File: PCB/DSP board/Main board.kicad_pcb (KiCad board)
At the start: 4 copper layers, 60 x 100 mm, 208 parts, among them J201 01x06 male SMD, J701 Conn_01x40_Female, J702 Conn_01x06_Female, J801 1140084168, J901 USB_B, U201 STM32H743II, U401 AS4C32M8SA, U501 CS42448, U601 MIC23050, U602 TPS2113A, U603 TPS61170, U604 ADP150, U901 USB3300-EZK, X101 Mini_PCI-e, Y201 ABS05-32.768, Y202 CX2016DB16000, Y901 XRCGB24M000F1H02R0

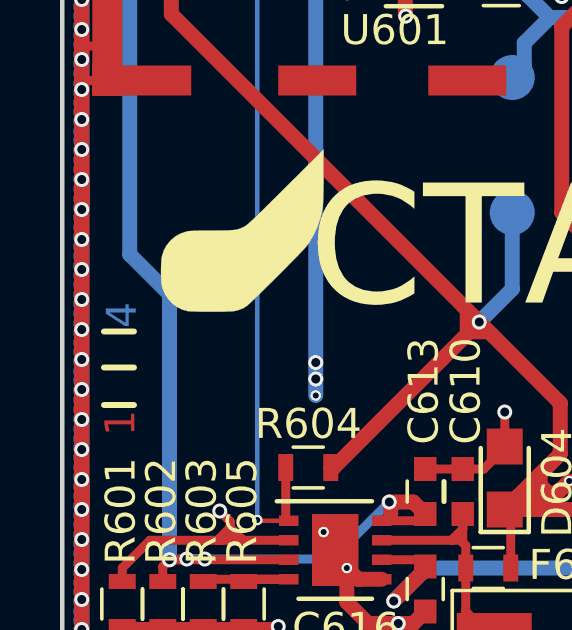
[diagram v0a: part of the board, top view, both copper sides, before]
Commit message: Minor updates keepout
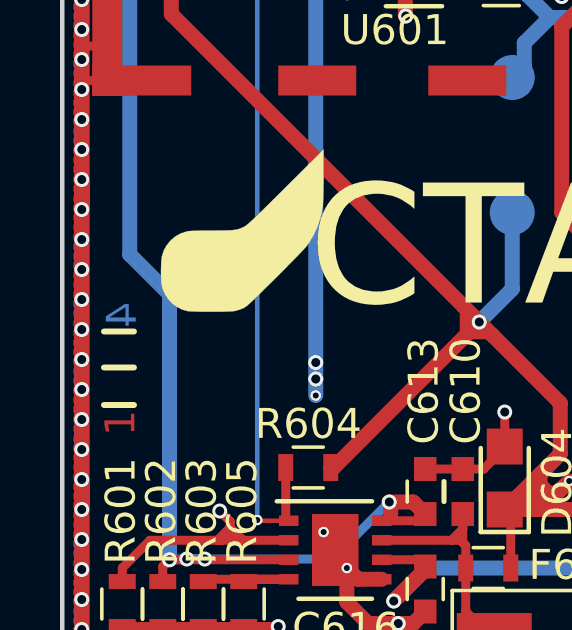
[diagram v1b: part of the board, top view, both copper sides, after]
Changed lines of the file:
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@@
   (layers
     (0 F.Cu mixed)
-    (1 In1.Cu mixed hide)
+    (1 In1.Cu mixed)
     (2 In2.Cu mixed)
     (31 B.Cu mixed)
@@
     (trace_clearance 0.1524)
     (zone_clearance 0.508)
-    (zone_45_only no)
+    (zone_45_only yes)
     (trace_min 0.1524)
     (segment_width 0.2)
@@
   (gr_line (start 198.790901 111.515901) (end 197.790901 111.515901) (angle 90) (layer F.SilkS) (width 0.2))
   (gr_text 4 (at 198.390901 108.5159 90) (layer B.Cu)
-    (effects (font (size 1 1) (thickness 0.2)))
+    (effects (font (size 1 1) (thickness 0.2)) (justify mirror))
   )
   (gr_text 3 (at 198.340901 109.665901 90) (layer In2.Cu)
-    (effects (font (size 1 1) (thickness 0.2)))
+    (effects (font (size 1 1) (thickness 0.2)) (justify mirror))
   )
   (gr_text 2 (at 198.340901 110.865901 90) (layer In1.Cu)
@@
       )
     )
+  )
+  (zone (net 0) (net_name "") (layer In1.Cu) (hatch edge 0.508)
+    (connect_pads yes (clearance 0.508))
+    (min_thickness 0.254)
+    (keepout (tracks not_allowed) (vias not_allowed) (copperpour not_allowed))
+    (fill (arc_segments 16) (thermal_gap 0.508) (thermal_bridge_width 0.508))
+    (polygon
+      (pts
+        (xy 197.65 108.05) (xy 198.95 108.05) (xy 198.95 112.55) (xy 197.65 112.55)
+      )
+    )
+  )
+  (zone (net 0) (net_name "") (layer F.Cu) (hatch edge 0.508)
+    (connect_pads yes (clearance 0.508))
+    (min_thickness 0.254)
+    (keepout (tracks not_allowed) (vias not_allowed) (copperpour not_allowed))
+    (fill (arc_segments 16) (thermal_gap 0.508) (thermal_bridge_width 0.508))
+    (polygon
+      (pts
+        (xy 197.65 108.05) (xy 198.95 108.05) (xy 198.95 112.55) (xy 197.65 112.55)
+      )
+    )
+  )
+  (zone (net 0) (net_name "") (layer In2.Cu) (hatch edge 0.508)
+    (connect_pads yes (clearance 0.508))
+    (min_thickness 0.254)
+    (keepout (tracks not_allowed) (vias not_allowed) (copperpour not_allowed))
+    (fill (arc_segments 16) (thermal_gap 0.508) (thermal_bridge_width 0.508))
+    (polygon
+      (pts
+        (xy 197.65 108.05) (xy 198.95 108.05) (xy 198.95 112.55) (xy 197.65 112.55)
+      )
+    )
+  )
+  (zone (net 0) (net_name "") (layer B.Cu) (hatch edge 0.508)
+    (connect_pads yes (clearance 0.508))
+    (min_thickness 0.254)
+    (keepout (tracks not_allowed) (vias not_allowed) (copperpour not_allowed))
+    (fill (arc_segments 16) (thermal_gap 0.508) (thermal_bridge_width 0.508))
+    (polygon
+      (pts
+        (xy 197.65 108.05) (xy 198.95 108.05) (xy 198.95 112.55) (xy 197.65 112.55)
+      )
+    )
